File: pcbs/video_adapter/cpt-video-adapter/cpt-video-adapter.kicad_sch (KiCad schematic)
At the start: 4 parts, among them J1 Conn_02x05_Odd_Even, J2 cpt-backplane_100, U1 mc10125

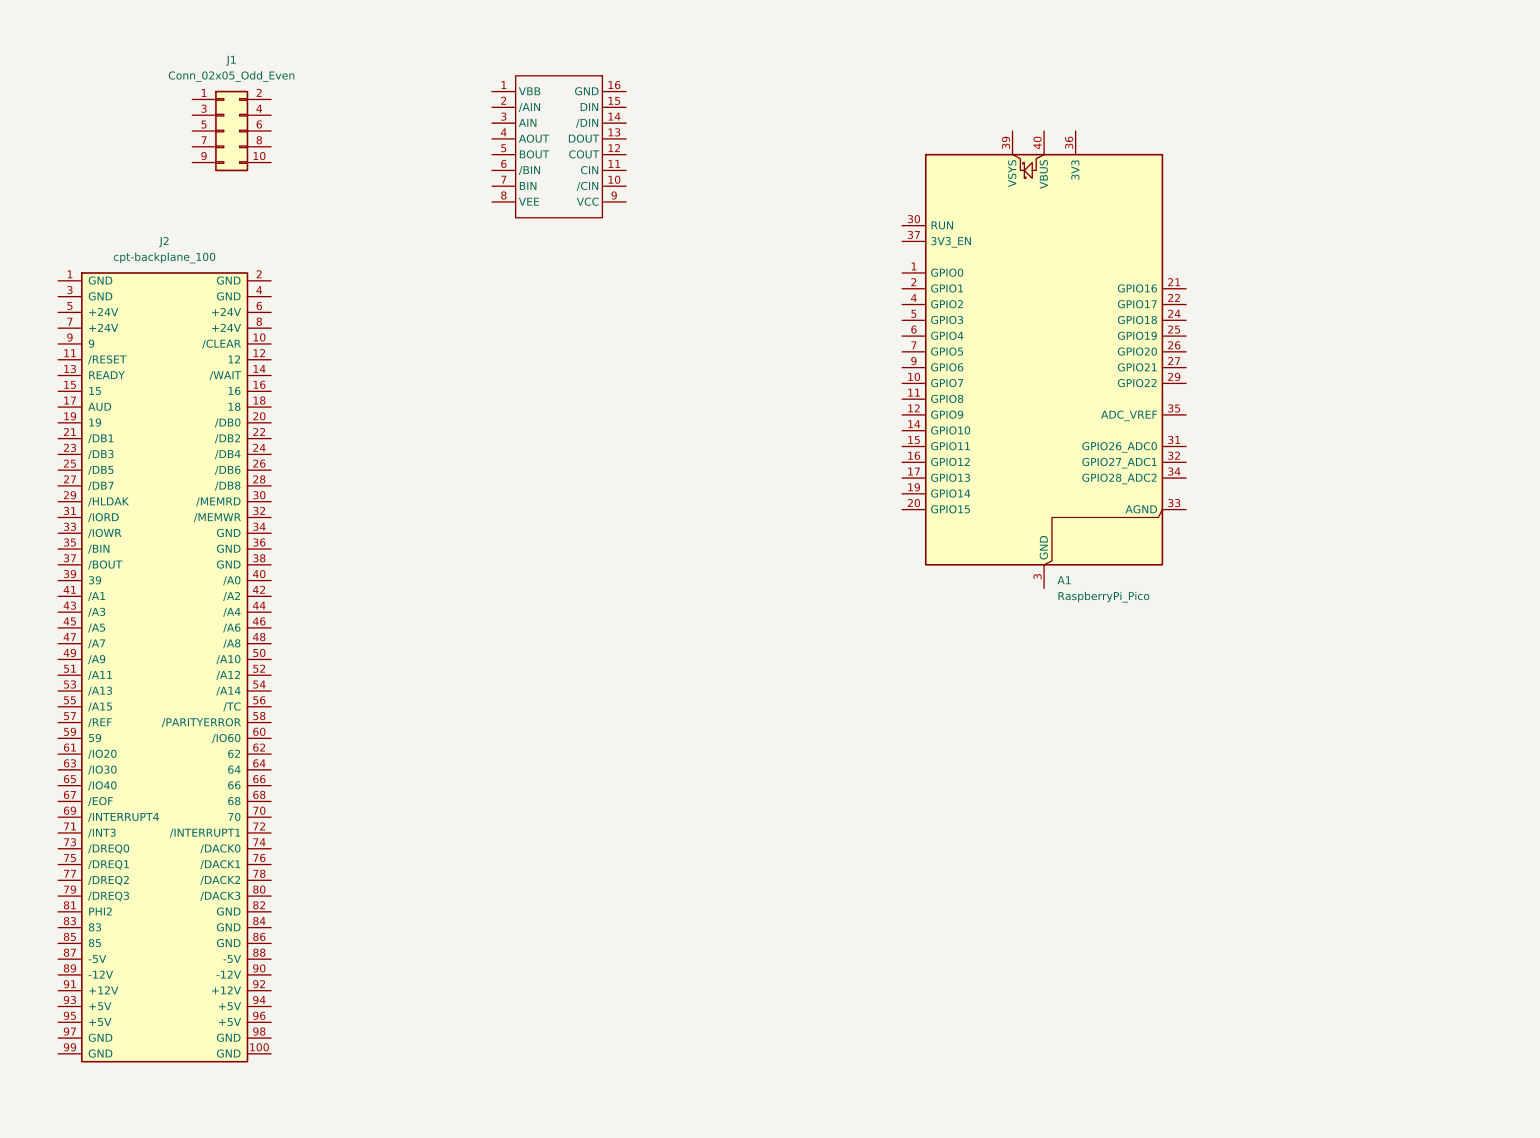
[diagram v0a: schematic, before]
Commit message: "Update"
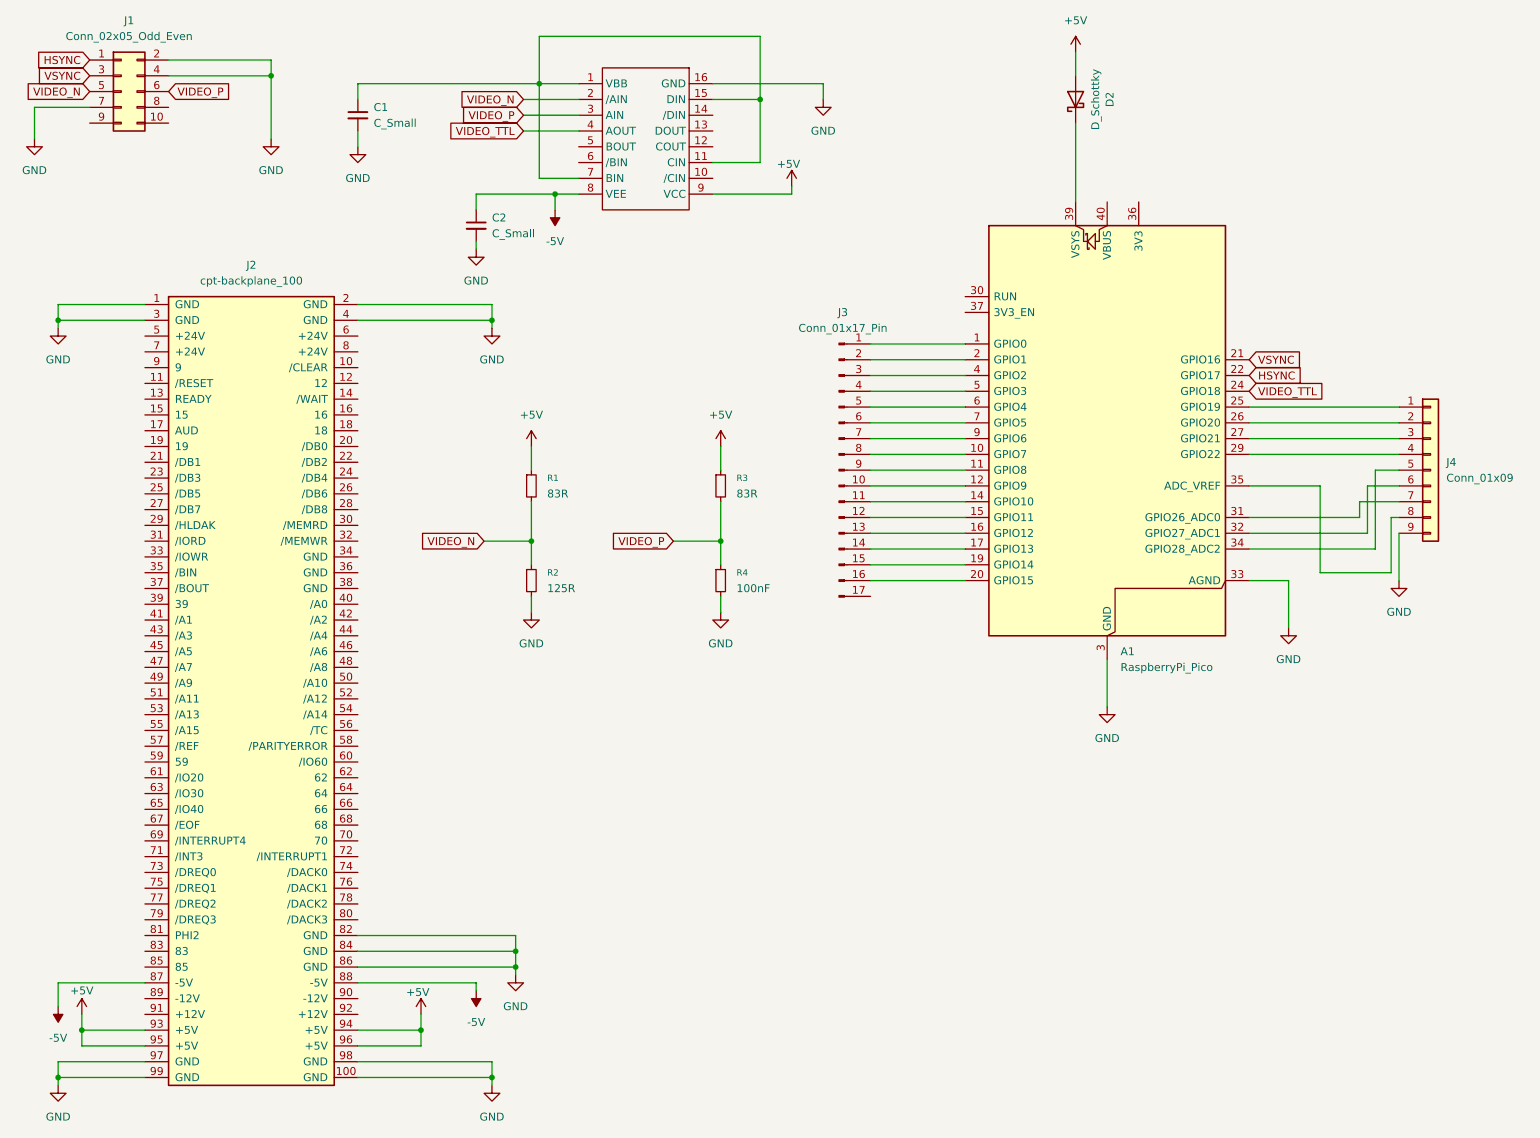
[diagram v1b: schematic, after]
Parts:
- added C1, C2: C_Small, Capacitor_SMD:C_0805_2012Metric_Pad1.18x1.45mm_HandSolder, symbol Device:C_Small
- added D2: D_Schottky, Diode_SMD:D_SOD-123, symbol Device:D_Schottky
- added J3: Conn_01x17_Pin, Connector_PinHeader_2.54mm:PinHeader_1x17_P2.54mm_Vertical, symbol Connector:Conn_01x17_Pin
- added J4: Conn_01x09, Connector_PinSocket_2.54mm:PinSocket_1x09_P2.54mm_Vertical, symbol Connector_Generic:Conn_01x09
- added R1, R3: 83R, Resistor_SMD:R_0805_2012Metric_Pad1.20x1.40mm_HandSolder, symbol Device:R_Small
- added R2: 125R, Resistor_SMD:R_0805_2012Metric_Pad1.20x1.40mm_HandSolder, symbol Device:R_Small
- added R4: 100nF, Resistor_SMD:R_0805_2012Metric_Pad1.20x1.40mm_HandSolder, symbol Device:R_Small
- J1: KiLib_Generator (none) -> connector/pin_header_socket
- J2: footprint ajm-cpt:cpt-card-edge-100 -> ajm-video:cpt-card-edge-100
- U1: footprint (none) -> Package_DIP:DIP-16_W7.62mm
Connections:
- net GND: now reaches J2.1 (GND)
- net GND: now also A1.13 (GND), A1.18 (GND), A1.23 (GND), A1.28 (GND), A1.3 (GND), A1.33 (AGND), A1.38 (GND), A1.8 (GND), J1.2 (Pin_2), J1.4 (Pin_4), J1.7 (Pin_7), J2.100 (GND), J2.2 (GND), J2.3 (GND), J2.4 (GND), J2.82 (GND), J2.84 (GND), J2.86 (GND), J2.97 (GND), J2.98 (GND), J2.99 (GND), U1.16 (GND), C1.2, C2.2, J4.9 (Pin_9), R2.2, R4.2
- net -5V: now reaches J2.87 (-5V)
- net -5V: now also J2.88 (-5V), U1.8 (VEE), C2.1
- net +5V: now reaches J2.93 (+5V)
- net +5V: now also J2.94 (+5V), J2.95 (+5V), J2.96 (+5V), U1.9 (VCC), D2.2 (A), R1.1, R3.1
- net at U1.1 (VBB): now also U1.11 (CIN), U1.15 (DIN), U1.7 (BIN), C1.1
- net VIDEO_N: now reaches U1.2 (/AIN)
- net VIDEO_N: now also J1.5 (Pin_5), R1.2, R2.1
- net VIDEO_P: now reaches U1.3 (AIN)
- net VIDEO_P: now also J1.6 (Pin_6), R3.2, R4.1
- net VIDEO_TTL: now reaches U1.4 (AOUT)
- net VIDEO_TTL: now also A1.24 (GPIO18)
- net at A1.1 (GPIO0): now also J3.1 (Pin_1)
- net at A1.10 (GPIO7): now also J3.8 (Pin_8)
- net at A1.11 (GPIO8): now also J3.9 (Pin_9)
- net at A1.12 (GPIO9): now also J3.10 (Pin_10)
- net at A1.14 (GPIO10): now also J3.11 (Pin_11)
- net at A1.15 (GPIO11): now also J3.12 (Pin_12)
- net at A1.16 (GPIO12): now also J3.13 (Pin_13)
- net at A1.17 (GPIO13): now also J3.14 (Pin_14)
- net at A1.19 (GPIO14): now also J3.15 (Pin_15)
- net at A1.2 (GPIO1): now also J3.2 (Pin_2)
- net at A1.20 (GPIO15): now also J3.16 (Pin_16)
- net VSYNC: now reaches A1.21 (GPIO16)
- net VSYNC: now also J1.3 (Pin_3)
- net HSYNC: now reaches A1.22 (GPIO17)
- net HSYNC: now also J1.1 (Pin_1)
- net at A1.25 (GPIO19): now also J4.1 (Pin_1)
- net at A1.26 (GPIO20): now also J4.2 (Pin_2)
- net at A1.27 (GPIO21): now also J4.3 (Pin_3)
- net at A1.29 (GPIO22): now also J4.4 (Pin_4)
- net at A1.31 (GPIO26_ADC0): now also J4.7 (Pin_7)
- net at A1.32 (GPIO27_ADC1): now also J4.6 (Pin_6)
- net at A1.34 (GPIO28_ADC2): now also J4.5 (Pin_5)
- net at A1.35 (ADC_VREF): now also J4.8 (Pin_8)
- net at A1.39 (VSYS): now also D2.1 (K)
- net at A1.4 (GPIO2): now also J3.3 (Pin_3)
- net at A1.5 (GPIO3): now also J3.4 (Pin_4)
- net at A1.6 (GPIO4): now also J3.5 (Pin_5)
- net at A1.7 (GPIO5): now also J3.6 (Pin_6)
- net at A1.9 (GPIO6): now also J3.7 (Pin_7)
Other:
- moved on the sheet: A1, J1, J2
